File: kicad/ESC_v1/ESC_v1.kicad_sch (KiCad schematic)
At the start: 52 parts, among them J1 Conn_01x05_Pin, J10 Conn_01x01_Pin, J11 Conn_01x01_Pin, J12 Conn_01x01_Pin, J13 Conn_01x03_Pin, J14 Conn_01x01_Pin, J15 Conn_01x01_Pin, J16 Conn_01x01_Pin, J17 Conn_01x04_Pin, J2 Conn_01x05_Pin, J3 Conn_01x03_Pin, J4 Conn_01x03_Pin, J5 Conn_01x01_Pin, J6 Conn_01x06_Pin, J8 Conn_01x04_Pin, U10 BD4104, U11 ADuM1201AR, U12 ACS711xEXLT-15AB, U19 STM32G431CBUx, U8 ACS711xEXLT-15AB, U9 ACS711xEXLT-15AB

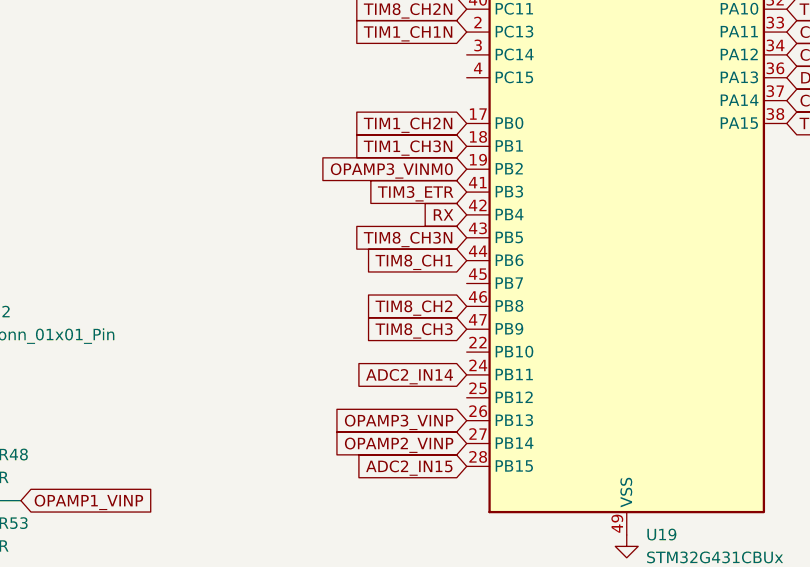
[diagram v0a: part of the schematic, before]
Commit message: a
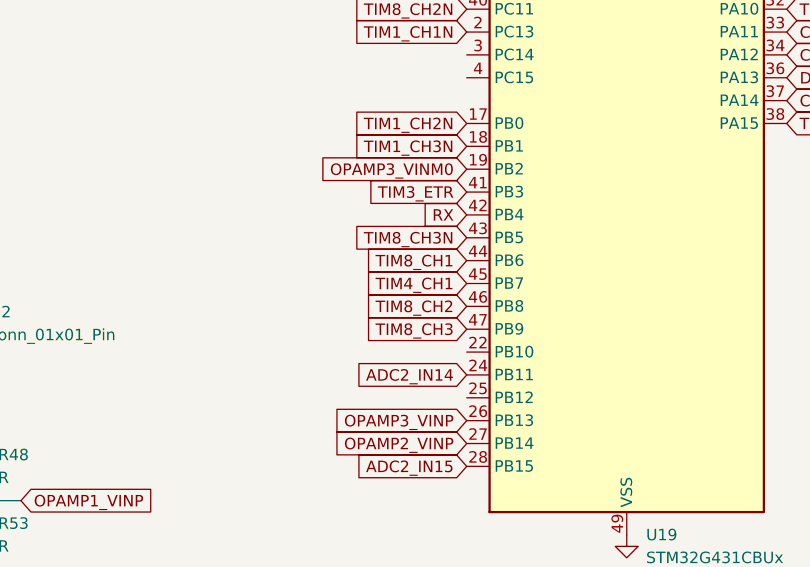
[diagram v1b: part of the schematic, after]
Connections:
- net TIM4_CH1: now also U19.45 (PB7)
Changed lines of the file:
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@@
+		)
+	)
+	(global_label "TIM4_CH1"
+		(shape input)
+		(at 180.34 107.95 180)
+		(fields_autoplaced yes)
+		(effects
+			(font
+				(size 1.27 1.27)
+			)
+			(justify right)
+		)
+		(property "Intersheetrefs" "${INTERSHEET_REFS}"
+			(at 168.3439 107.95 0)
+			(effects
+				(font
+					(size 1.27 1.27)
+				)
+				(justify right)
+				(hide yes)
+			)
 		)
 	)
